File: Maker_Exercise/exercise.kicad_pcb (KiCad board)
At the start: 2 copper layers, 35 parts, among them J1 USB_C_Receptacle_USB2.0_16P, J2 Conn_01x02, J3 Conn_ST_STDC14, J4 Conn_01x04, U1 USBLC6-2SC6, U2 STM32G431CBUx

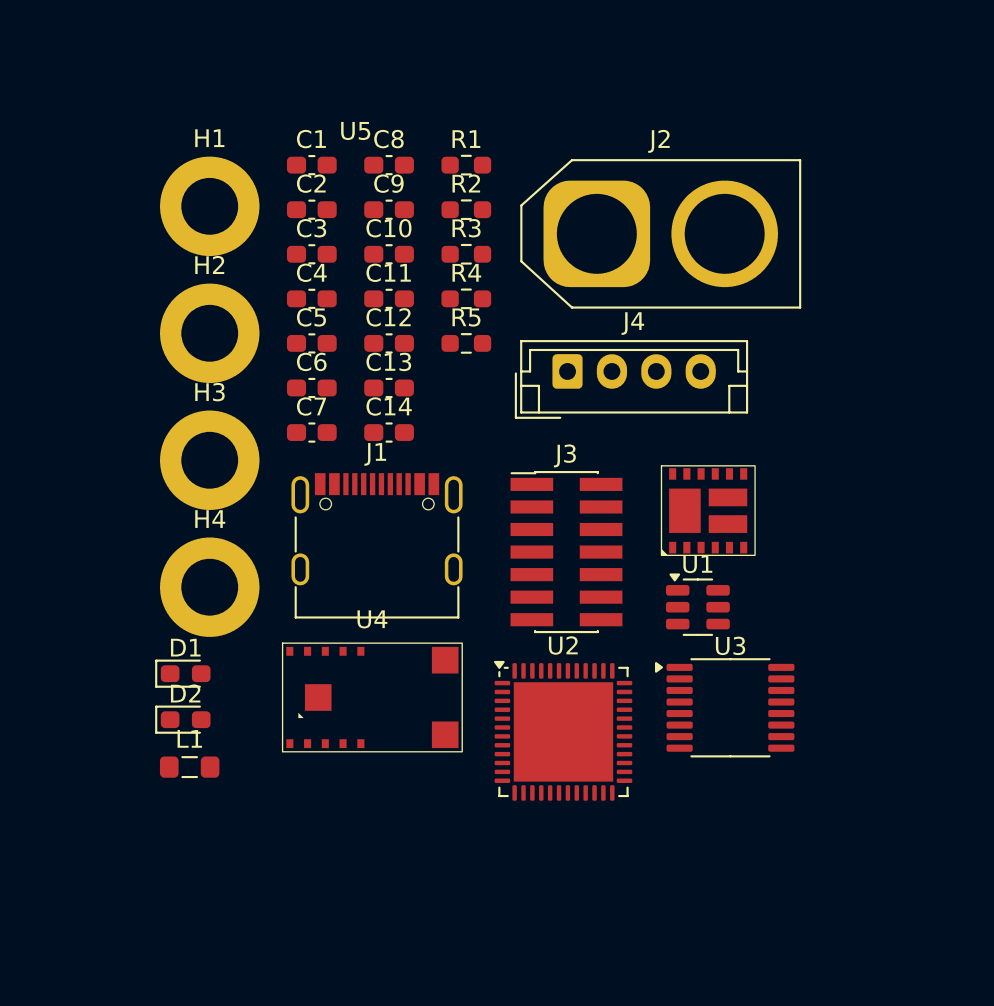
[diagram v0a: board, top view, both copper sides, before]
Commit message: finalized PCB and routing
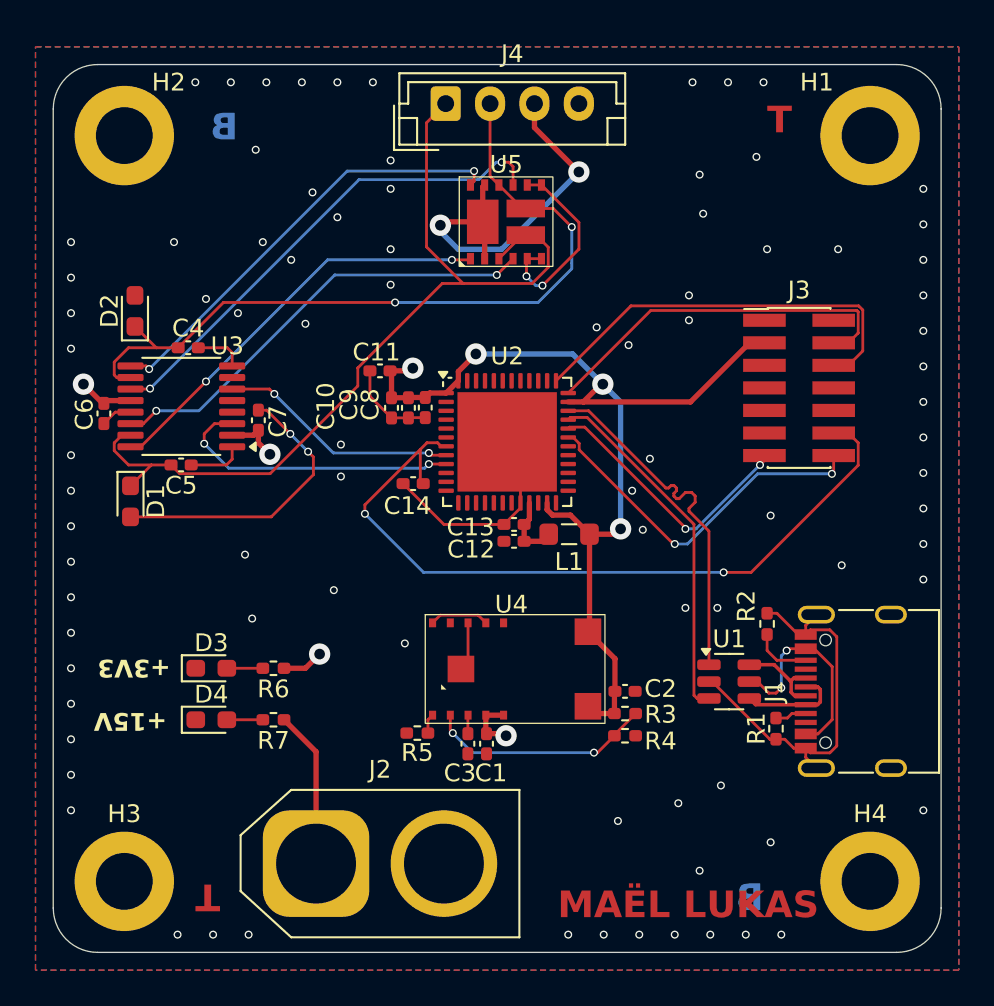
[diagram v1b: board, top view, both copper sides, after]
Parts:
- added D3: LED_Small, LED_SMD:LED_0603_1608Metric_Pad1.05x0.95mm_HandSolder, F.Cu at (135.9, 91.0)
- added D4: LED_Small, LED_SMD:LED_0603_1608Metric_Pad1.05x0.95mm_HandSolder, F.Cu at (135.9, 93.9)
- added R6: 820, Resistor_SMD:R_0402_1005Metric_Pad0.72x0.64mm_HandSolder, F.Cu at (139.4, 91.0)
- added R7: 5k6, Resistor_SMD:R_0402_1005Metric_Pad0.72x0.64mm_HandSolder, F.Cu at (139.4, 93.9)
- C1, C10, C11, C12, C13, C14, C2, C3, C4, C5, C6, C7, C8, C9: footprint Capacitor_SMD:C_0603_1608Metric_Pad1.08x0.95mm_HandSolder -> Capacitor_SMD:C_0402_1005Metric_Pad0.74x0.62mm_HandSolder
- R1, R2, R3, R4, R5: footprint Resistor_SMD:R_0603_1608Metric_Pad0.98x0.95mm_HandSolder -> Resistor_SMD:R_0402_1005Metric_Pad0.72x0.64mm_HandSolder
- moved H4 40.7 mm to (173.0, 103.0)
- moved J2 38.8 mm to (141.8, 102.0)
- moved H1 37.4 mm to (173.0, 61.0)
- moved R1 36.2 mm to (167.7, 94.4), turned to -90 degrees
- moved U3 35.3 mm to (134.2, 76.2), turned to 180 degrees
- moved C1 34.0 mm to (151.4, 95.2), turned to -90 degrees
- moved C2 32.4 mm to (159.2, 92.3)
- moved J1 29.0 mm to (173.1, 92.3), turned to 90 degrees
- moved C3 28.9 mm to (150.3, 95.2), turned to -90 degrees
- moved R2 28.8 mm to (167.2, 88.5), turned to 90 degrees
- moved R3 27.4 mm to (159.2, 93.5)
- moved R4 26.2 mm to (159.2, 94.8)
- moved L1 25.1 mm to (156.1, 83.5), turned to 180 degrees
- moved H3 24.2 mm to (131.0, 103.0)
- moved D2 23.2 mm to (131.6, 70.9), turned to 90 degrees
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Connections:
- U1 pad 1: D+ -> USB_DP
- U1 pad 3: USB_DP -> USB_DM
- U1 pad 4: USB_DM -> D-
- U1 pad 6: D- -> D+
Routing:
- net GND: track 0.00 -> 71.8 mm, vias 0 -> 91
- net +3V3: track 0.00 -> 59.3 mm, vias 0 -> 5
- net S1/D2_Drive: track 0.00 -> 49.8 mm
- net D3/S4_Drive: track 0.00 -> 44.3 mm, vias 0 -> 2
- net NRST: track 0.00 -> 43.1 mm, vias 0 -> 2
- net +15V: track 0.00 -> 40.4 mm, vias 0 -> 5
- net G3_Drive: track 0.00 -> 28.0 mm, vias 0 -> 2
- net G2_Drive: track 0.00 -> 25.4 mm, vias 0 -> 2
- net G4_Drive: track 0.00 -> 24.9 mm, vias 0 -> 2
- net G1_Drive: track 0.00 -> 23.5 mm, vias 0 -> 2
- net SWCLK: track 0.00 -> 23.4 mm
- net SWDIO: track 0.00 -> 21.1 mm
- net UART_DEBUG_TX: track 0.00 -> 20.3 mm, vias 0 -> 2
- net USB_DM: track 0.00 -> 20.2 mm
- net USB_DP: track 0.00 -> 20.1 mm
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- added copper zone on In2.Cu, net +15V
- added copper zone on In2.Cu, net +3V3
- added copper zone on B.Cu, net GND
- added copper zone on F.Cu, net GND
- added copper zone on In1.Cu, net GND
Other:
- board outline added: 50 x 50 mm
- copper layers 2 -> 4
- board text added: "+15V"
- board text added: "+3V3"
- board text added: "B"
- board text added: "MAËL LUKAS"
- board text added: "T"
